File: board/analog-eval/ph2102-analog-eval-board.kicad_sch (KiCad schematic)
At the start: 41 parts, among them J1 CONN_PROBE, U1 LMC662, U2 TLV2333, U3 REF3020, U4 MCP3201-BI/SN, U5 LM27762

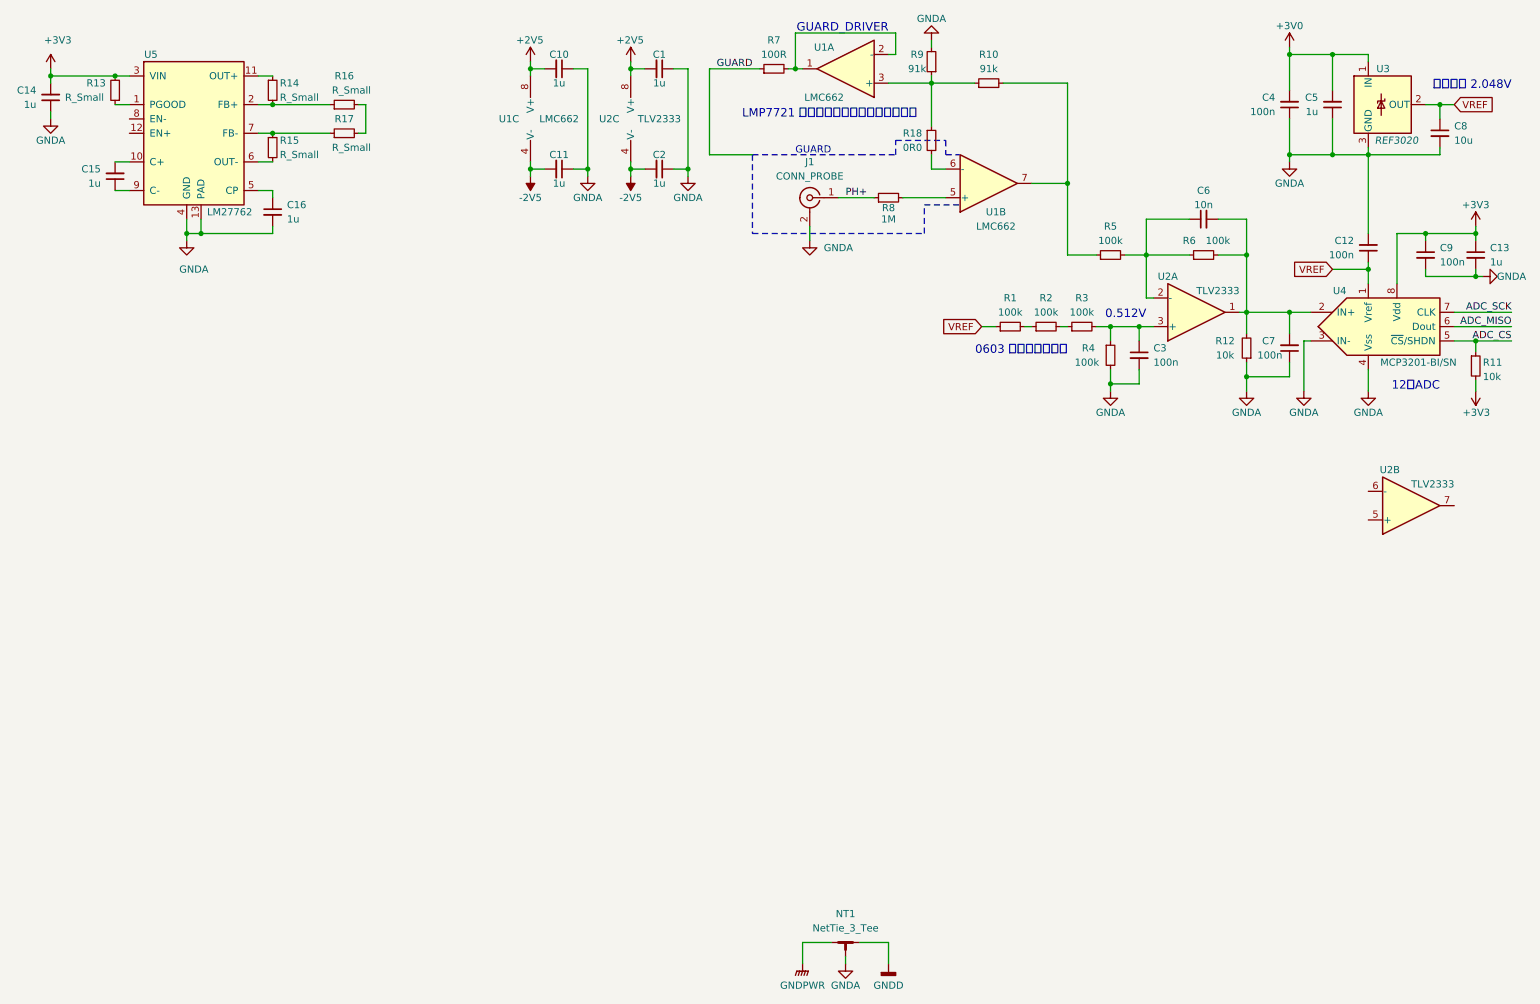
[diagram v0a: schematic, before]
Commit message: update
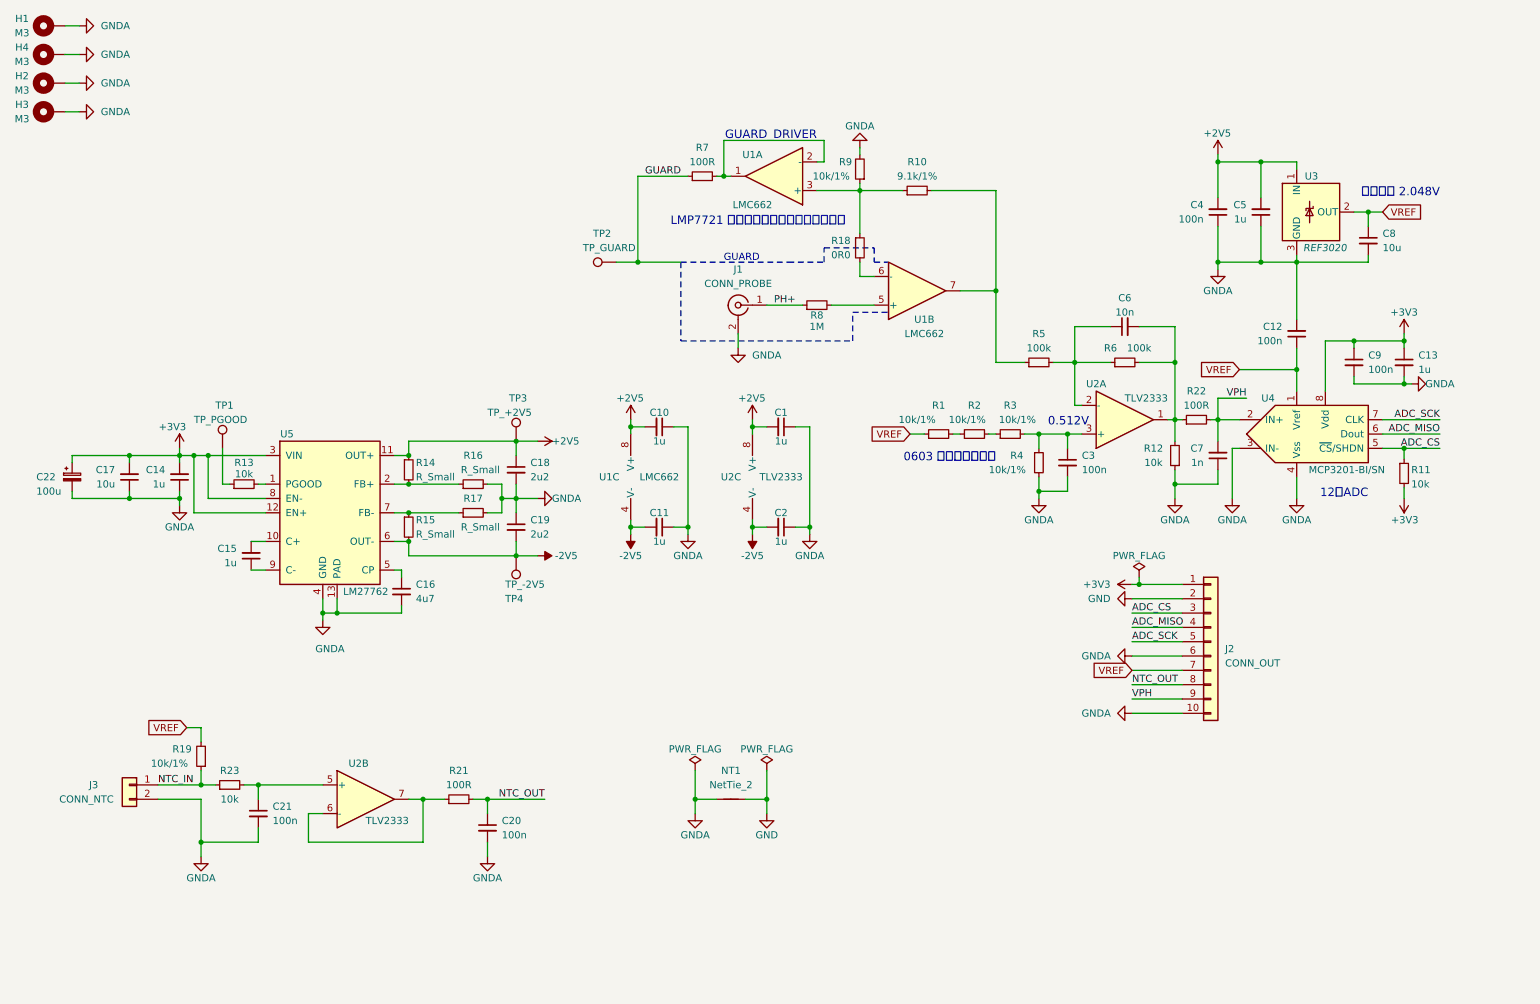
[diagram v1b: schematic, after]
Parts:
- removed NT1: NetTie_3_Tee, symbol Device:NetTie_3_Tee
- added C17: 10u, Capacitor_SMD:C_0603_1608Metric, symbol Device:C_Small
- added C18, C19: 2u2, Capacitor_SMD:C_0603_1608Metric, symbol Device:C_Small
- added C20, C21: 100n, Capacitor_SMD:C_0603_1608Metric, symbol Device:C_Small
- added C22: 100u, Capacitor_Tantalum_SMD:CP_EIA-3528-15_AVX-H, symbol Device:C_Polarized_Small
- added H1, H2, H3, H4: M3, MountingHole:MountingHole_3.2mm_M3_Pad_Via, symbol Mechanical:MountingHole_Pad
- added J2: CONN_OUT, Connector_PinHeader_2.54mm:PinHeader_1x10_P2.54mm_Vertical, symbol Connector_Generic:Conn_01x10
- added J3: CONN_NTC, Connector_JST:JST_XH_S2B-XH-A-1_1x02_P2.50mm_Horizontal, symbol Connector_Generic:Conn_01x02
- added NT1: NetTie_2, NetTie:NetTie-2_SMD_Pad2.0mm, symbol Device:NetTie_2
- added R19: 10k/1%, Resistor_SMD:R_0603_1608Metric, symbol Device:R_Small
- added R21, R22: 100R, Resistor_SMD:R_0603_1608Metric, symbol Device:R_Small
- added R23: 10k, Resistor_SMD:R_0603_1608Metric, symbol Device:R_Small
- added TP1: TP_PGOOD, TestPoint:TestPoint_Pad_D1.0mm, symbol Connector:TestPoint
- added TP2: TP_GUARD, symbol Connector:TestPoint
- added TP3: TP_+2V5, TestPoint:TestPoint_Pad_D1.0mm, symbol Connector:TestPoint
- added TP4: TP_-2V5, TestPoint:TestPoint_Pad_D1.0mm, symbol Connector:TestPoint
- C1, C10, C11, C12, C13, C14, C15, C2, C3, C4, C5, C6, C8, C9: footprint (none) -> Capacitor_SMD:C_0603_1608Metric
- C16: value 1u -> 4u7; footprint (none) -> Capacitor_SMD:C_0603_1608Metric
- C7: value 100n -> 1n; footprint (none) -> Capacitor_SMD:C_0603_1608Metric
- J1: footprint (none) -> Connector_Coaxial:BNC_Amphenol_B6252HB-NPP3G-50_Horizontal
- R1, R2, R3, R4: value 100k -> 10k/1%; footprint (none) -> Resistor_SMD:R_0603_1608Metric
- R10: value 91k -> 9.1k/1%; footprint (none) -> Resistor_SMD:R_0603_1608Metric
- R11, R12, R14, R15, R16, R17, R5, R6, R8: footprint (none) -> Resistor_SMD:R_0603_1608Metric
- R13: value R_Small -> 10k; footprint (none) -> Resistor_SMD:R_0603_1608Metric
- R18: footprint Resistor_SMD:R_0805_2012Metric -> Resistor_SMD:R_1206_3216Metric_Pad1.30x1.75mm_HandSolder
- R7: footprint Resistor_SMD:R_0402_1005Metric -> Resistor_SMD:R_0603_1608Metric
- R9: value 91k -> 10k/1%; footprint (none) -> Resistor_SMD:R_0603_1608Metric
- U2, U4: footprint (none) -> Package_SO:SOIC-8_3.9x4.9mm_P1.27mm
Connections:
- net +3V0 is gone; now on net +2V5: C4.2, C5.2, U3.1 (IN)
- net +2V5: now also R14.1, U5.11 (OUT+), C18.1, TP3.1
- net +3V3: now also U5.12 (EN+), U5.8 (EN-), C17.2, C22.1, J2.1 (Pin_1); no longer R13.2
- net -2V5: now also R15.2, U5.6 (OUT-), C19.2, TP4.1
- net ADC_CS: now also J2.3 (Pin_3)
- net ADC_MISO: now also J2.4 (Pin_4)
- net ADC_SCK: now also J2.5 (Pin_5)
- net GNDA: now also R16.2, R17.2, C17.1, C18.2, C19.1, C20.2, C21.2, C22.2, H1.1, H2.1, H3.1, H4.1, J2.10 (Pin_10), J2.6 (Pin_6), J3.2 (Pin_2), NT1.1
- net GUARD: now also TP2.1
- net VREF: now also J2.7 (Pin_7), R19.2
- net at C6.2, R12.2, R6.2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: now also R22.1; no longer C7.2, U4.2 (IN+)
- net at R13.1: now also TP1.1; no longer U5.1 (PGOOD)
- net at U2.5 (+): now also C21.1, R23.2
- net at U2.6 (-): now also U2.7, R21.1
- new net: R13.2, U5.1 (PGOOD)
- new net GND: J2.2 (Pin_2), NT1.2
- new net NTC_IN: J3.1 (Pin_1), R19.1, R23.1
- new net NTC_OUT: C20.1, J2.8 (Pin_8), R21.2
- new net VPH: C7.2, J2.9 (Pin_9), R22.2, U4.2 (IN+)
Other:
- moved on the sheet: C1, C10, C11, C12, C13, C14, C15, C16, C2, C3, C4, C5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
